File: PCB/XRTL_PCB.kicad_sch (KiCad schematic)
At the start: 20 parts, among them J1 POWER, J10 servo1, J11 servo2, J12 infoLED, J2 stepper1, J3 stepper2, J4 ESP32 right, J5 ESP32 left, K1 TIANBO-HJR-4102-L, K2 TIANBO-HJR-4102-L, U1 TBD62003, U2 TBD62003

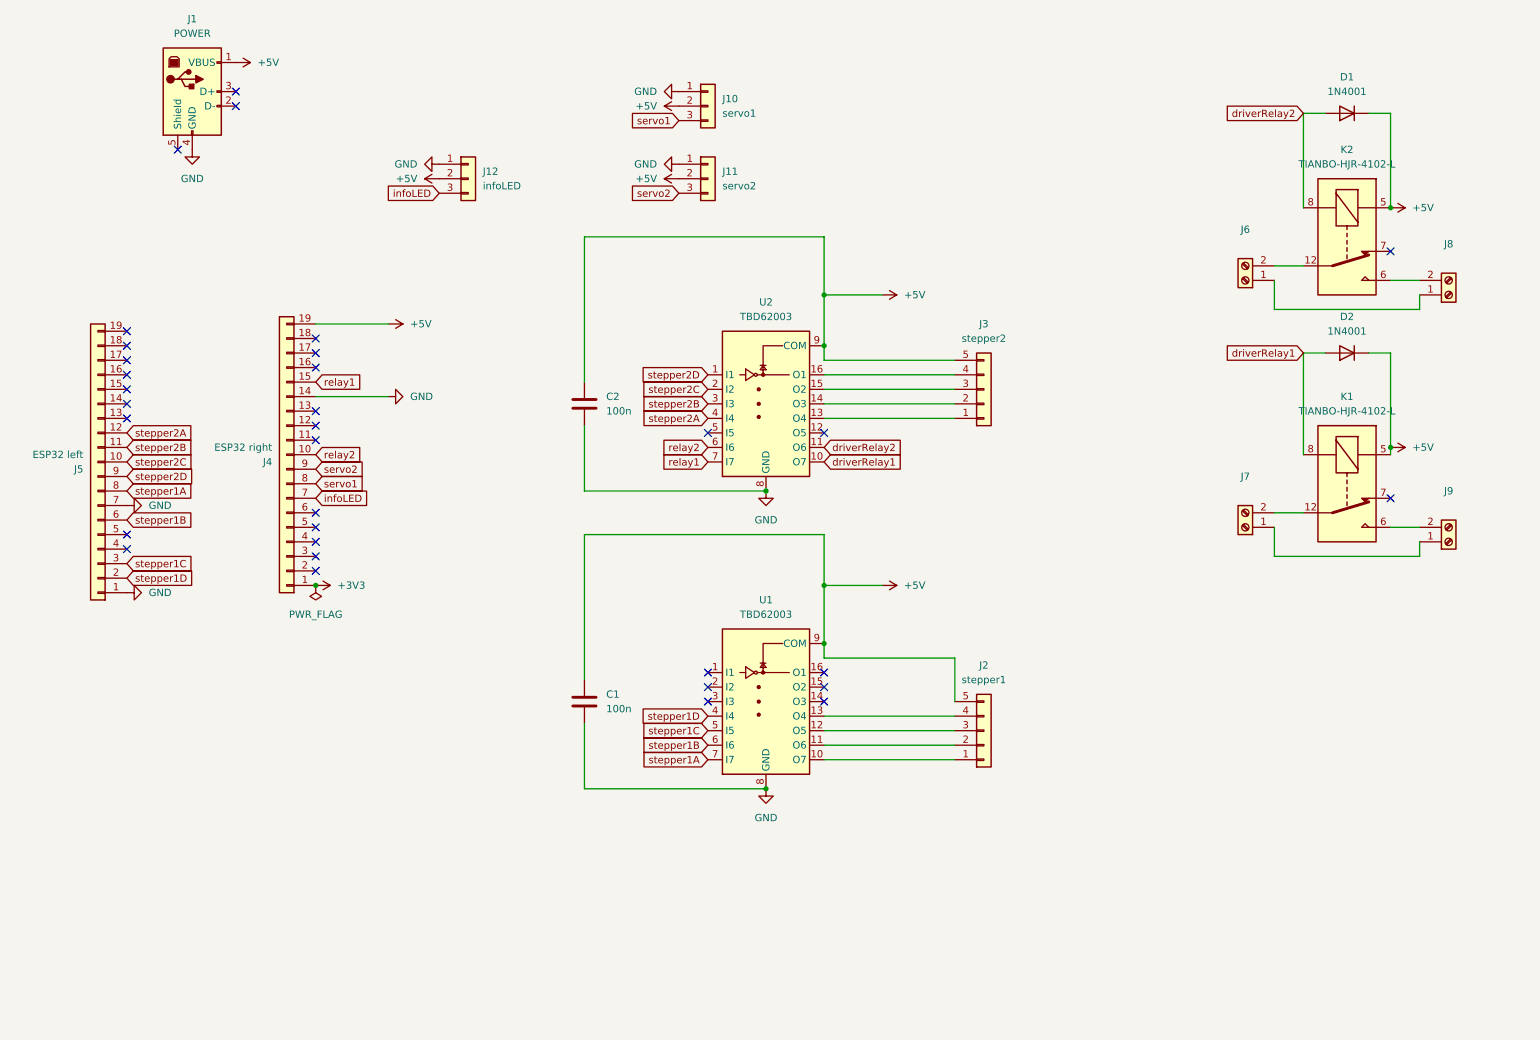
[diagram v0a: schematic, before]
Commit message: Add files via upload
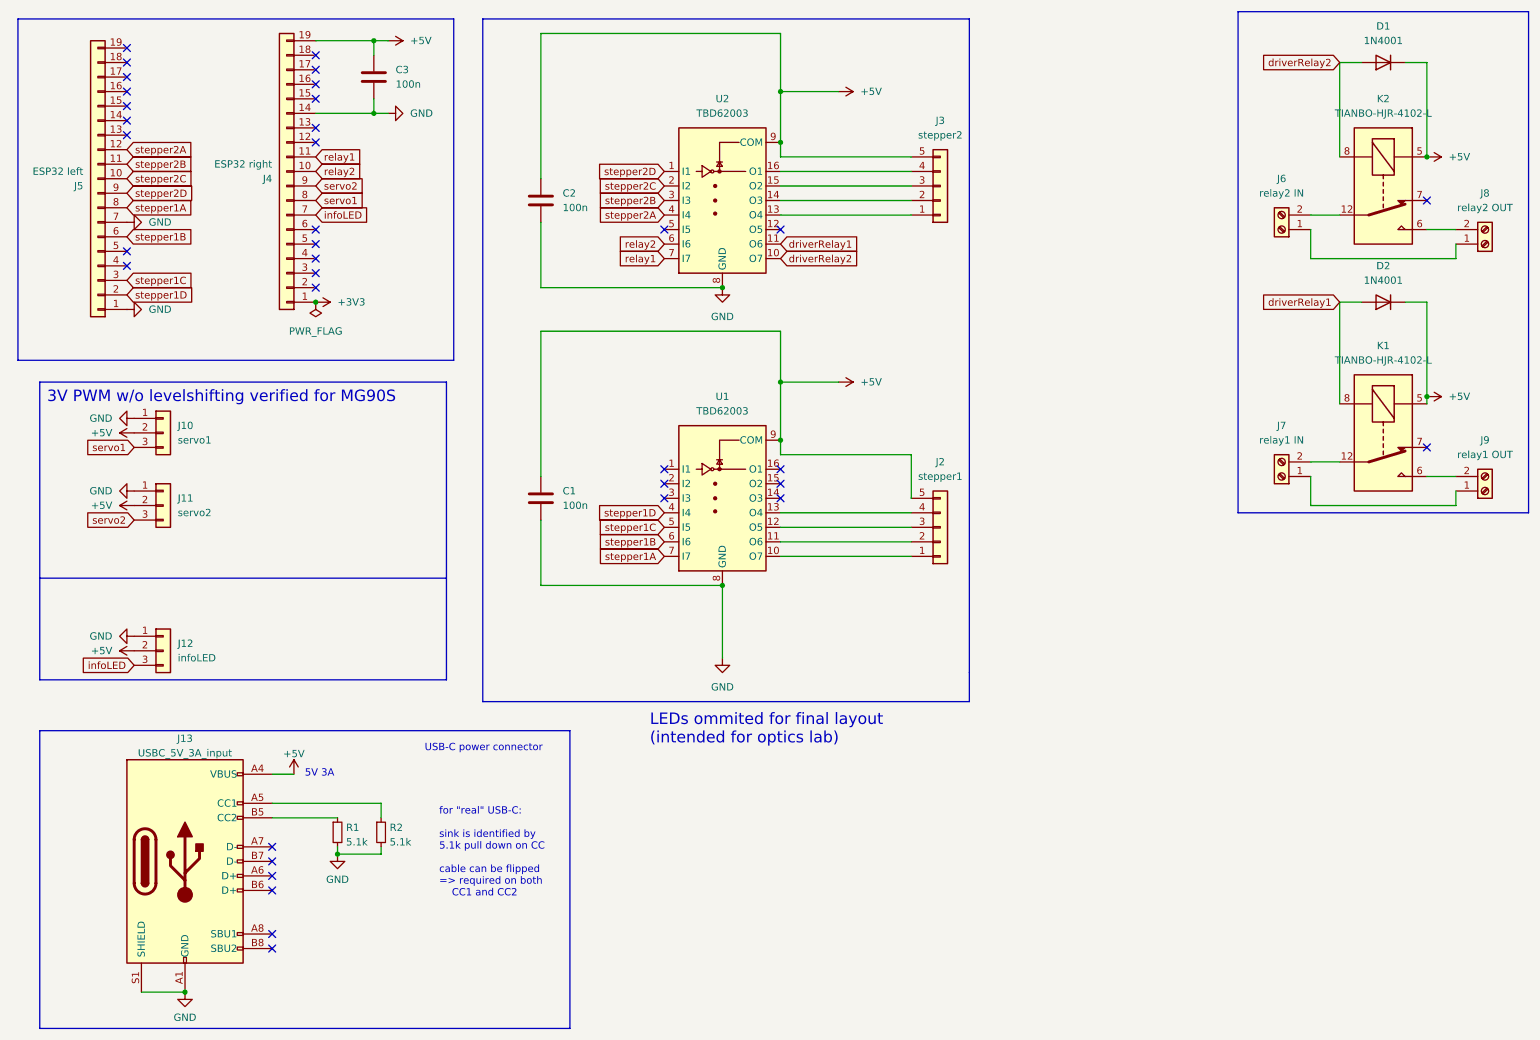
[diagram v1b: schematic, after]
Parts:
- removed J1: POWER, Connector_USB:USB_A_Stewart_SS-52100-001_Horizontal, symbol Connector:USB_B
- added C3: 100n, Capacitor_THT:C_Disc_D3.0mm_W1.6mm_P2.50mm, symbol Device:C
- added J13: USBC_5V_3A_input, Connector_USB:USB_C_Receptacle_GCT_USB4085, symbol Connector:USB_C_Receptacle_USB2.0
- added R1, R2: 5.1k, Resistor_THT:R_Axial_DIN0204_L3.6mm_D1.6mm_P5.08mm_Horizontal, symbol Device:R_Small
- C1, C2: footprint Capacitor_THT:C_Disc_D3.4mm_W2.1mm_P2.50mm -> Capacitor_THT:C_Disc_D3.0mm_W1.6mm_P2.50mm
- J6: value (none) -> relay2 IN
- J7: value (none) -> relay1 IN
- J8: value (none) -> relay2 OUT; footprint (none) -> TerminalBlock_Phoenix:TerminalBlock_Phoenix_MKDS-1,5-2-5.08_1x02_P5.08mm_Horizontal
- J9: value (none) -> relay1 OUT
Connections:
- net +5V: now also C3.1, J13.A4 (VBUS), J13.A9 (VBUS), J13.B4 (VBUS), J13.B9 (VBUS)
- net GND: now also C3.2, J13.A1 (GND), J13.A12 (GND), J13.B1 (GND), J13.B12 (GND), J13.S1 (SHIELD), R1.2, R2.2
- net driverRelay1: now also U2.11 (O6); no longer U2.10 (O7)
- net driverRelay2: now also U2.10 (O7); no longer U2.11 (O6)
- net relay1: now also J4.11 (Pin_11); no longer J4.15 (Pin_15)
- new net: J13.A5 (CC1), R2.1
- new net: J13.B5 (CC2), R1.1
- no-connect marks 33 -> 36
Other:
- note added: "3V PWM w/o levelshifting verified for MG90S"
- note added: "5V 3A"
- note added: "LEDs ommited for final layout (intended for optics lab)"
- note added: "USB-C power connector"
- note added: "for "real" USB-C: sink is identified by 5.1k pull down on CC cable can be flipped => required on both CC1 and CC2"
- title: (none) -> XR Twin Lab
- moved on the sheet: C1, C2, D1, D2, J10, J11, J12, J2, J3, J4, J5, J6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
